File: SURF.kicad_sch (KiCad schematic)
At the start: 73 parts, among them Q1 BC338, Q2 BC338, Q3 Q_Dual_PMOS_S1G1D2S2G2D1, Q4 BC338, SW1 SW_MEC_5E, SW3 SW_MEC_5E, U1 ESP32-S2-MINI-2, U10 COMM_10_RIGHT, U11 CONN_10_LEFT, U2 CP2102N-A02-GQFN28, U3 SK68XXMINI-HS, U5 MICRO USB, U6 NCP164CSN300T1G, U7 XC6206PxxxMR, U8 XC6206PxxxMR, U9 LED_FLASH

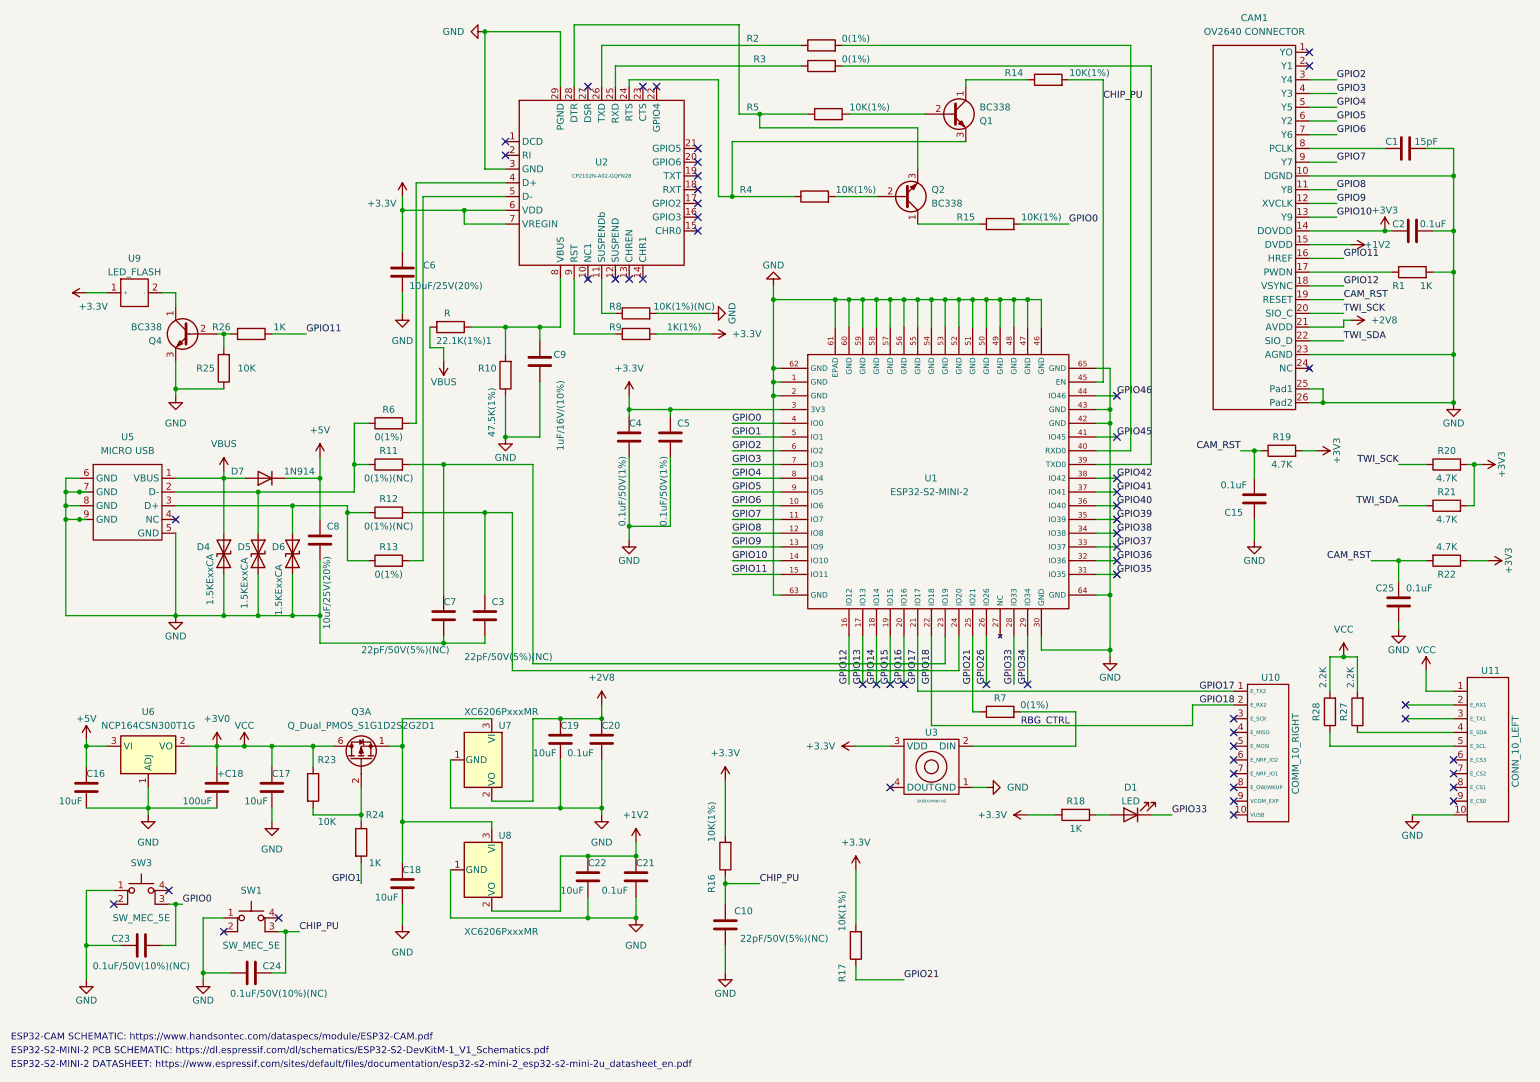
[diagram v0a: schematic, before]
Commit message: new
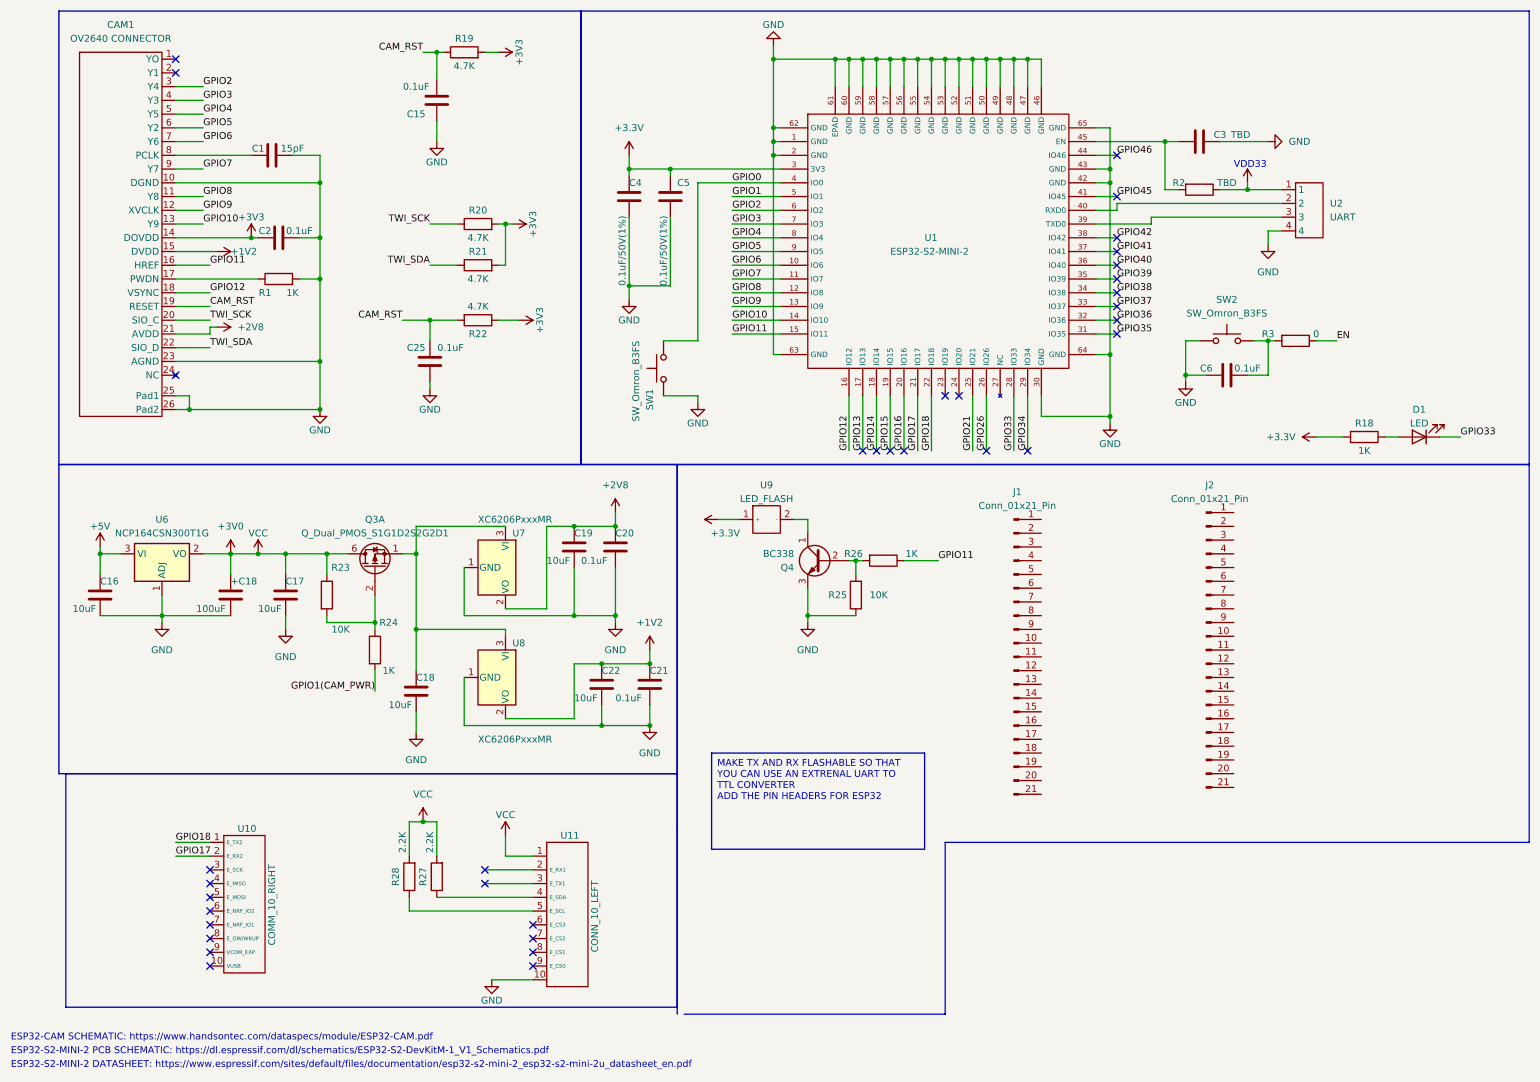
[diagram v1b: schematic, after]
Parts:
- removed 22.1K(1%)1: R, symbol Device:R
- removed C10, C7: 22pF/50V(5%)(NC), symbol Device:C
- removed C23, C24: 0.1uF/50V(10%)(NC), symbol Device:C
- removed C8: 10uF/25V(20%), symbol Device:C
- removed C9: 1uF/16V/(10%), symbol Device:C
- removed D4, D5, D6: 1.5KExxCA, Diode_THT:D_DO-201AE_P15.24mm_Horizontal, symbol Diode:1.5KExxCA
- removed D7: 1N914, Diode_THT:D_DO-35_SOD27_P7.62mm_Horizontal, symbol Diode:1N914
- removed Q1, Q2: BC338, Package_TO_SOT_THT:TO-92_Inline, symbol Transistor_BJT:BC338
- removed R10: 47.5K(1%), symbol Device:R
- removed R11, R12: 0(1%)(NC), symbol Device:R
- removed R13, R6, R7: 0(1%), symbol Device:R
- removed R14, R15, R16, R17, R4, R5: 10K(1%), symbol Device:R
- removed R8: 10K(1%)(NC), symbol Device:R
- removed R9: 1K(1%), symbol Device:R
- removed SW1, SW3: SW_MEC_5E, symbol Switch:SW_MEC_5E
- removed U2: CP2102N-A02-GQFN28, CP2102N-A02-GQFN28:QFN50P500X500X80-29N, symbol CP2102N:CP2102N-A02-GQFN28
- removed U3: SK68XXMINI-HS, SK6812MINI:SK6812MINI, symbol New:SK68XXMINI
- removed U5: MICRO USB, new:1051640001, symbol New_2:Micro_USB
- added J1, J2: Conn_01x21_Pin, symbol Connector:Conn_01x21_Pin
- added SW1, SW2: SW_Omron_B3FS, symbol Switch:SW_Omron_B3FS
- added U2: UART, symbol New:UART
- C3: value 22pF/50V(5%)(NC) -> TBD
- C6: value 10uF/25V(20%) -> 0.1uF
- R2: value 0(1%) -> TBD
- R3: value 0(1%) -> 0
- U1: footprint (none) -> new:ESP32-S2-MINI-2
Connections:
- net CHIP_PU is gone; now on an unnamed net: U1.45 (EN)
- net +3.3V: no longer C6.1
- net GND: now also C3.1, SW1.1, SW2.1, U2.4; no longer C3.2
- net GPIO0: now also SW1.2
- net GPIO1: no longer R24.2
- net GPIO17: now also U10.2 (E_RX2); no longer U10.1 (E_TX2)
- net GPIO18: now also U10.1 (E_TX2); no longer U10.2 (E_RX2)
- net at U1.24 (IO20): no longer C3.1
- net EN: now reaches R3.1
- net at U1.39 (TXD0): now also U2.3; no longer R3.2
- net VDD: now reaches R2.1
- net VDD: now also U2.1
- net at R2.2: now also C3.2; no longer U1.40 (RXD0)
- new net: U1.40 (RXD0), U2.2
- new net: C6.1, R3.2, SW2.2
- new net GPIO1(CAM_PWR): R24.2
- no-connect marks 55 -> 35
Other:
- note added: "VDD33"
- note removed: "RBG_CTRL"
- moved on the sheet: +C18, C1, C15, C16, C17, C18, C19, C2, C20, C21, C22, C25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
